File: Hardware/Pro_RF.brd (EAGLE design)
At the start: 40.6 x 27.9 mm, 102 parts, among them U1 MCP73831, U2 915MHz, U5 ATmega32U4, U6 3.3V, Y2 8MHz

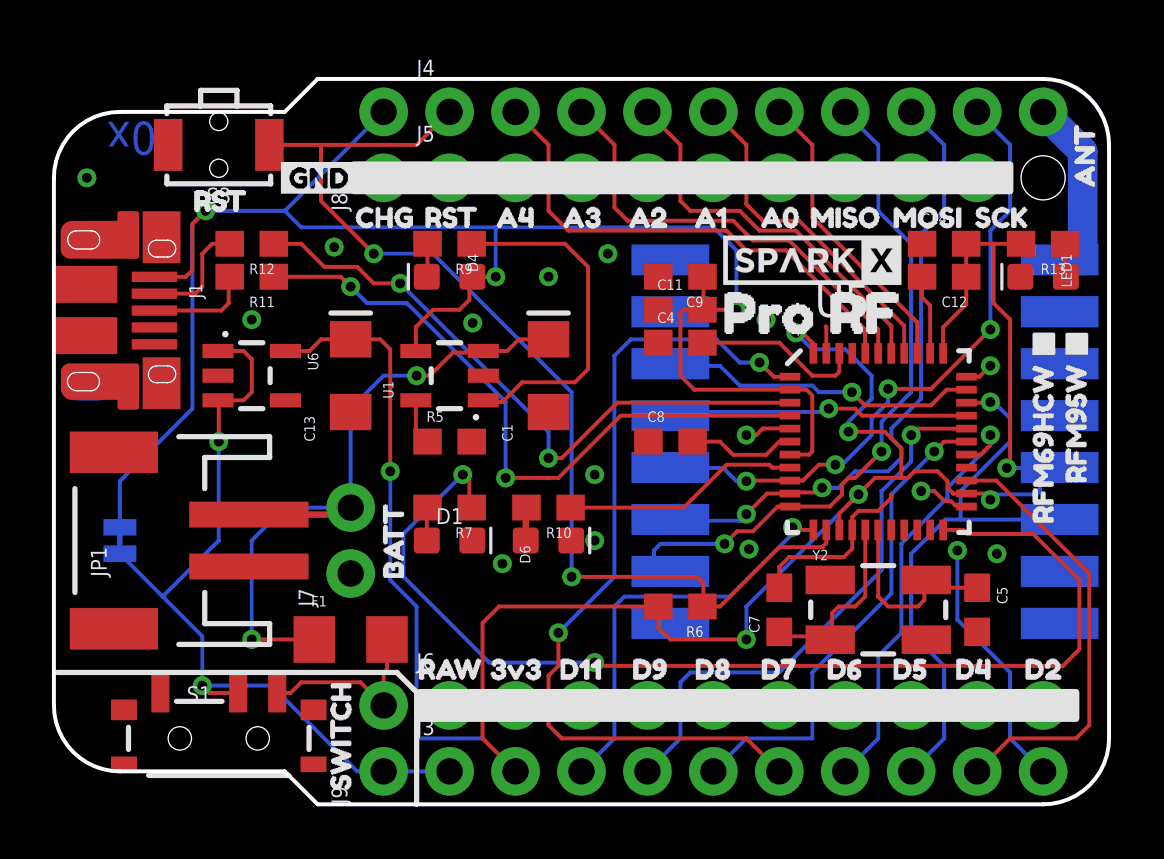
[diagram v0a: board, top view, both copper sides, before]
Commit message: Many updates. v02.
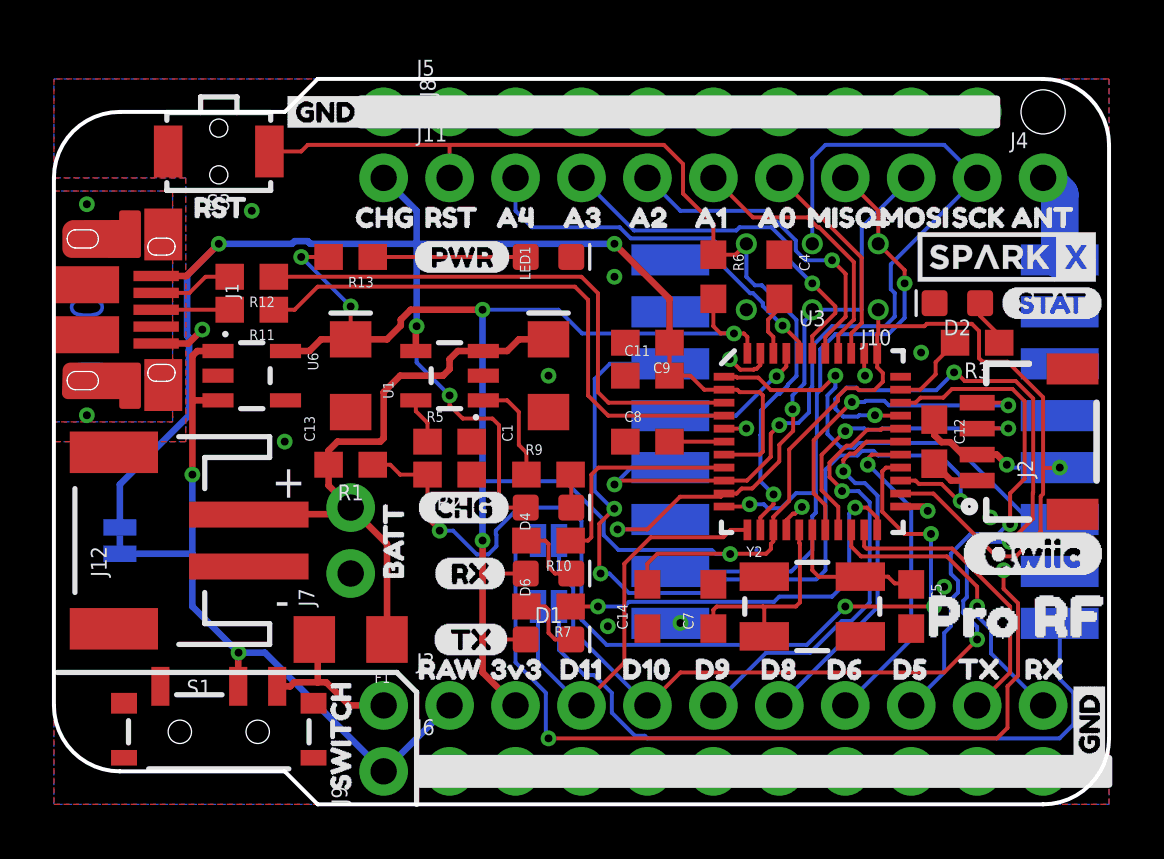
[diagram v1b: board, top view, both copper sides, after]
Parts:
- removed U$61: (no value), buzzard_labels (25):D212
- removed U5: ATmega32U4, SparkFun-IC-Microcontroller:QFN-44-NOPAD
- added D2: BLUE, SparkFun-LED:LED-0603
- added J10: AVR_SPI_PROG_3X2TESTPOINTS, SparkFun-Connectors:2X3_TEST_POINTS
- added J11: (no value), SparkFun-Connectors:1X09_NO_SILK
- added J12: JST, SparkFun-Connectors:JST-2-SMD
- added J2: (no value), SparkFun-Connectors:1X04_1MM_RA
- added JP2: (no value), SparkFun-Jumpers:SMT-JUMPER_2_NO_SILK
- added R1, R2: 10k, SparkFun-Resistors:0603
- added R3: 1k, SparkFun-Resistors:0603
- added U$62: (no value), buzzard_labels (25):GND0
- added U$63: (no value), Labels:PWR-()-03
- added U$65: (no value), buzzard_labels (9):CHG1
- added U$66: (no value), Labels:QWIIC-()-04
- added U$68: (no value), buzzard_labels (9):D100
- added U$69: (no value), buzzard_labels (8):TX3
- added U$70: (no value), buzzard_labels (8):TX6
- added U$71: (no value), buzzard_labels (8):STAT5
- added U$72: (no value), buzzard_labels (8):RX7
- added U$73: (no value), buzzard_labels (8):RX2
- added U$74: (no value), buzzard_labels (25):D514
- added U3: 32U4, SparkFun-IC-Microcontroller:QFN-44-NOPAD
- D1: value GREEN -> Green
- D6: value BLUE -> Yellow
- J4: device SparkFun-Connectors:1X10_NO_SILK -> SparkFun-Connectors:1X01_NO_SILK
- J7: value (none) -> PTH
- J9: value (none) -> External On/Off
- JP1: device SparkFun-Connectors:JST-2-SMD -> SparkFun-Jumpers:SMT-JUMPER_2_NO_SILK
- SJ2: device SparkFun:SJ_2S-TRACE -> SparkFun-Jumpers:SMT-JUMPER_2_NC_TRACE_SILK
- U$15: device buzzard_labels (25):D212 -> buzzard_labels (10):D90
- U$16: device buzzard_labels (25):D413 -> buzzard_labels (10):D90
- U$17: device buzzard_labels (25):D514 -> buzzard_labels (25):GND0
- U$19: device buzzard_labels (25):D716 -> buzzard_labels (8):RX2
- U$21: device buzzard_labels (25):D918 -> buzzard_labels (9):D100
- U$25: device buzzard_labels (26):RFM69HCW_#0 -> buzzard_labels (3):LORA0
- U$26: value (none) -> SPECIAL_INSTRUCTIONS-ORDERING; device buzzard_labels (26):RFM95W_#1 -> SparkFun-Aesthetics:ORDERING_INSTRUCTIONS
- U$35: device buzzard_labels (25):RST2 -> buzzard_labels (3):WAN1
- U$55: device buzzard_labels (25):D918 -> buzzard_labels (25):D514
- U$57: device buzzard_labels (25):D716 -> buzzard_labels (8):TX3
- U$59: device buzzard_labels (25):D514 -> buzzard_labels (12):RFM69HCW#1
- U$60: device buzzard_labels (25):D413 -> buzzard_labels (12):RFM95W#0
- moved U$26 78.0 mm to (-34.3, -14.0), turned to 0 degrees
- moved R13 26.7 mm to (11.4, 21.1)
- moved J4 23.0 mm to (38.1, 24.1)
- moved U$25 22.3 mm to (15.9, 11.7), flipped to the bottom, turned to 270 degrees
- moved U$60 19.4 mm to (19.7, 13.7)
- moved LED1 19.1 mm to (19.1, 21.1), turned to 0 degrees
- moved C14 18.1 mm to (22.9, 7.62), turned to 90 degrees
- moved U$35 17.0 mm to (17.1, 11.7), flipped to the bottom, turned to 270 degrees
- moved U$59 16.0 mm to (22.2, 15.5)
- moved JP1 15.2 mm to (19.1, 10.2), flipped to the bottom, turned to 180 degrees
- moved U$51 15.2 mm to (2.54, 24.1)
- moved U$1 14.1 mm to (32.3, 7.24)
- moved U$19 13.1 mm to (39.6, 5.21), flipped to the bottom
- moved R6 12.8 mm to (25.4, 20.3), turned to 270 degrees
- moved U$15 12.7 mm to (24.0, 5.21)
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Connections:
- removed net A5: U5.41
- removed net D14: R10.1, U5.8
- removed net D2: J3.10
- removed net D4: J3.9, U5.25
- removed net D7: J3.6, U5.1
- removed net N$15: D1.A, R7.2
- removed net N$19: D6.A, R10.2
- removed net RST: J4.1, R6.1, S3.1, U5.13
- new net !CS: U2.5, U3.41
- new net !RST: J10.5, J11.1, R6.1, S3.1, U3.13
- new net D5: J3.8, U3.31
- new net N$1: D6.C, R10.2
- new net N$2: D1.C, R7.2
- new net N$3: D2.A, R3.1
- new net RFM_IO1: JP1.1, U2.15
- new net RFM_IO2: JP2.1, U2.16
- new net RXLED: R10.1, U3.8
- new net SHLD: J1.SHIELD, J1.SHIELD10, J1.SHIELD2, J1.SHIELD3, J1.SHIELD4, J1.SHIELD5, J1.SHIELD6, J1.SHIELD7, J1.SHIELD8, J1.SHIELD9
- new net STAT: R3.2, U3.32
- net 3.3V: now also D1.A, D6.A, J10.2, J2.2, U3.14, U3.24, U3.34, U3.44; no longer U5.14, U5.24, U5.34, U5.44
- net A0: now also J11.6, U3.36; no longer J4.6, U5.36
- net A1: now also J11.5, U3.37; no longer J4.5, U5.37
- net A2: now also J11.4, U3.38; no longer J4.4, U5.38
- net A3: now also J11.3, U3.39; no longer J4.3, U5.39
- net A4: now also J11.2, U3.40; no longer J4.2, U5.40
- net ANT: now also J4.1; no longer J4.10
- net AREF: now also U3.42; no longer U5.42
- net D+: now also U3.4; no longer U5.4
- net D-: now also U3.3; no longer U5.3
- net D10: now also J3.4, JP1.2, U3.30; no longer U2.5, U5.30
- net D11: now also JP2.2, U3.12; no longer U5.12
- net D6: now also U3.27; no longer U5.27
- net D8: now also J3.6, U3.28; no longer J3.5, U5.28
- net D9: now also J3.5, U3.29; no longer J3.4, U5.29
- net GND: now also D2.C, J10.6, J12.1, J2.1, R2.1, U3.15, U3.23, U3.33, U3.35, U3.43, U3.5; no longer D1.C, D6.C, JP1.1, U5.15, U5.23, U5.33, U5.35, U5.43, U5.5
- net MISO: now also J10.1, J11.7, U3.11; no longer J4.7, U5.11
- net MOSI: now also J10.4, J11.8, U3.10; no longer J4.8, U5.10
- net N$16: now also U3.16; no longer U5.16
- net N$17: now also U3.17; no longer U5.17
- net RFM_INT: now also U3.1; no longer J3.8, U5.31
- net RFM_RST: now also U3.25; no longer U5.32
- net RXI: now also J3.10, U3.20; no longer U5.20
- net SCK: now also J10.3, J11.9, U3.9; no longer J4.9, U5.9
- net SCL: now also J2.4, U3.18; no longer U5.18
- net SDA: now also J2.3, U3.19; no longer U5.19
- net TXLED: now also U3.22; no longer U5.22
- net TXO: now also J3.9, U3.21; no longer U5.21
- net UCAP: now also U3.6; no longer U5.6
- net USB_VCC: now also U3.2, U3.7; no longer U5.2, U5.7
- net VBATT: now also J12.2, R1.2; no longer JP1.2
- net VBATT_LVL: now also R1.1, R2.2, U3.26; no longer U5.26
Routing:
- net RST: track 41.8 -> 0.00 mm, vias 2 -> 0
- net VBATT_LVL: track 0.00 -> 37.8 mm, vias 0 -> 4
- net !RST: track 0.00 -> 36.1 mm, vias 0 -> 1
- net RFM_IO1: track 0.00 -> 35.4 mm, vias 0 -> 2
- net D10: track 11.6 -> 44.6 mm, vias 1 -> 4
- net D7: track 32.5 -> 0.00 mm, vias 2 -> 0
- net RFM_IO2: track 0.00 -> 27.7 mm
- net TXLED: track 42.7 -> 15.5 mm
- net RFM_RST: track 12.3 -> 34.1 mm, vias 1 -> 3
- net D5: track 0.00 -> 19.7 mm, vias 0 -> 1
- net D4: track 17.1 -> 0.00 mm
- net SCL: track 0.00 -> 13.1 mm, vias 0 -> 2
- net 3.3V: track 88.5 -> 101.4 mm, vias 7 -> 8
- net SDA: track 0.00 -> 12.0 mm, vias 0 -> 2
- net RXI: track 0.00 -> 11.8 mm, vias 0 -> 1
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- added copper zone on layer 1, net SHLD
- added copper zone on layer 16, net SHLD
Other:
- board text added: "+"
- board text added: "-"
- board text added: "0.8mm Board Thickness"
- board text added: "x02"
- board text removed: "x01"
